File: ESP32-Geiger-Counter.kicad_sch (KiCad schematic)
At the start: 55 parts, among them J1 USB_C_Receptacle_USB2.0_16P, Q1 Q_NPN_BCE, Q2 Q_NPN_BCE, SW1 SW_Push, SW2 SW_Push, U1 TP4056-42-ESOP8, U2 USBLC6-2SC6, U3 ESP32-WROOM-32, U4 TPS63031DSK, U5 Geiger Mueller Tube, U6 CP2102N-Axx-xQFN24, U7 MC34063AD

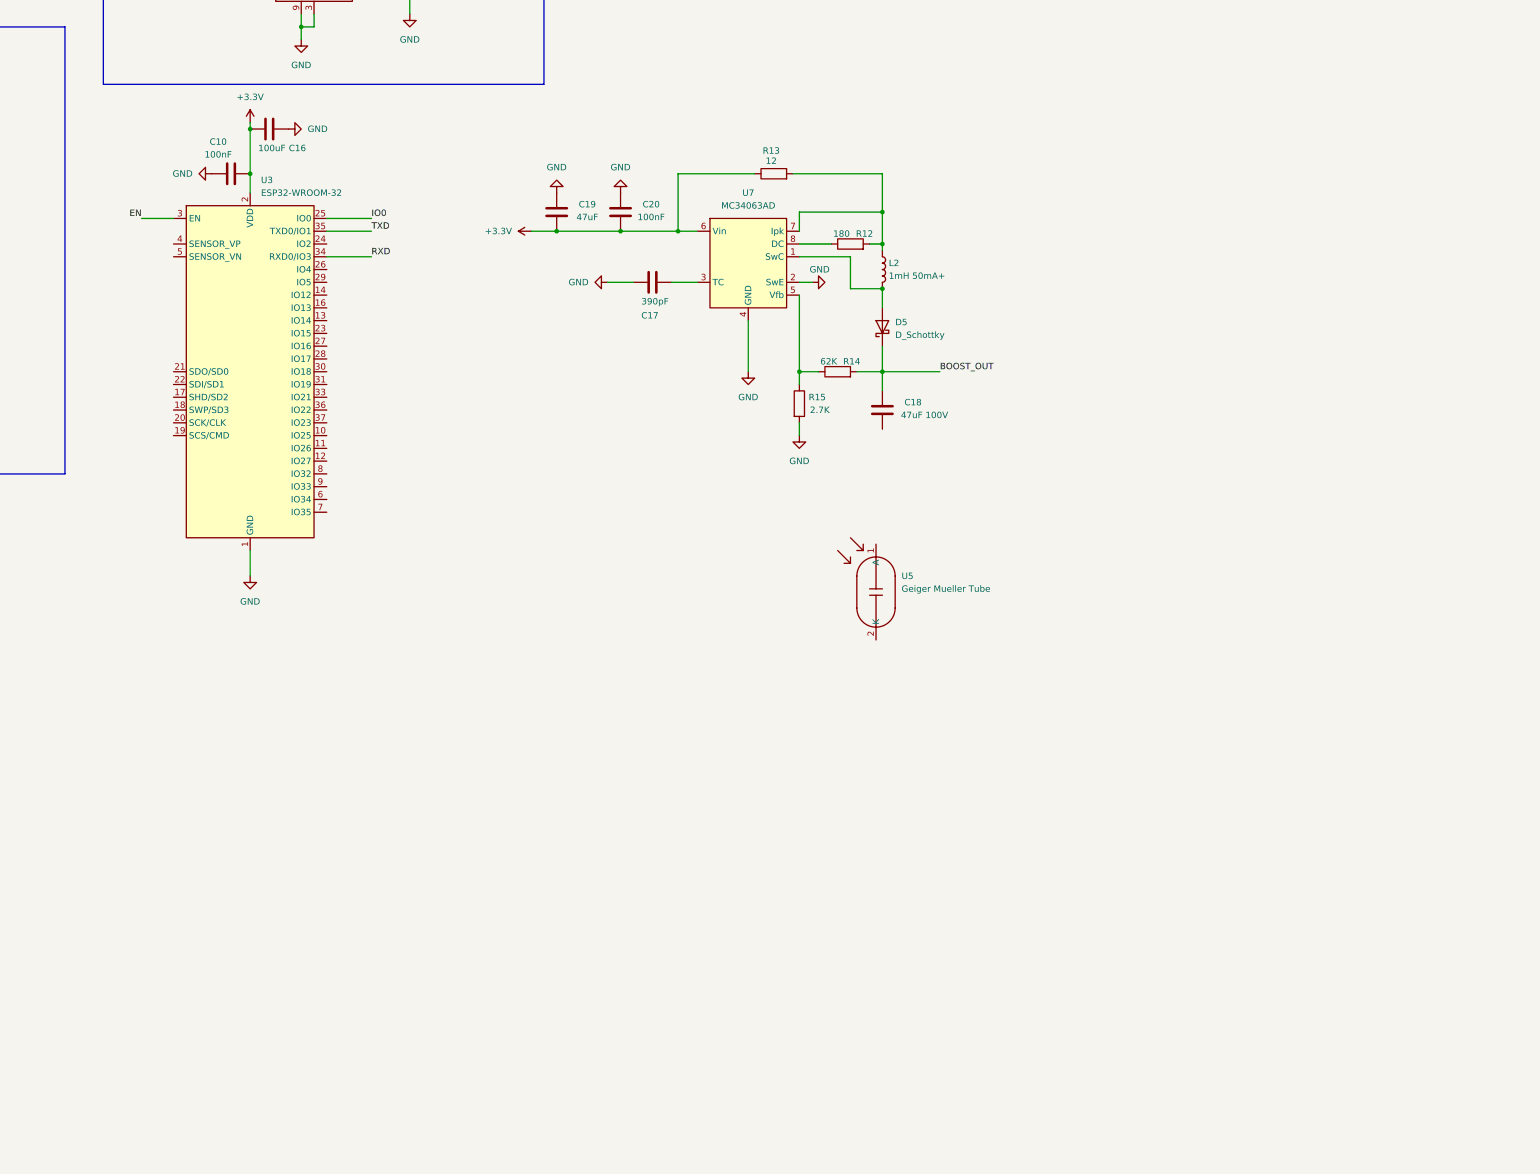
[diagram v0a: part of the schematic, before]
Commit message: idk if I will use this mega boost method
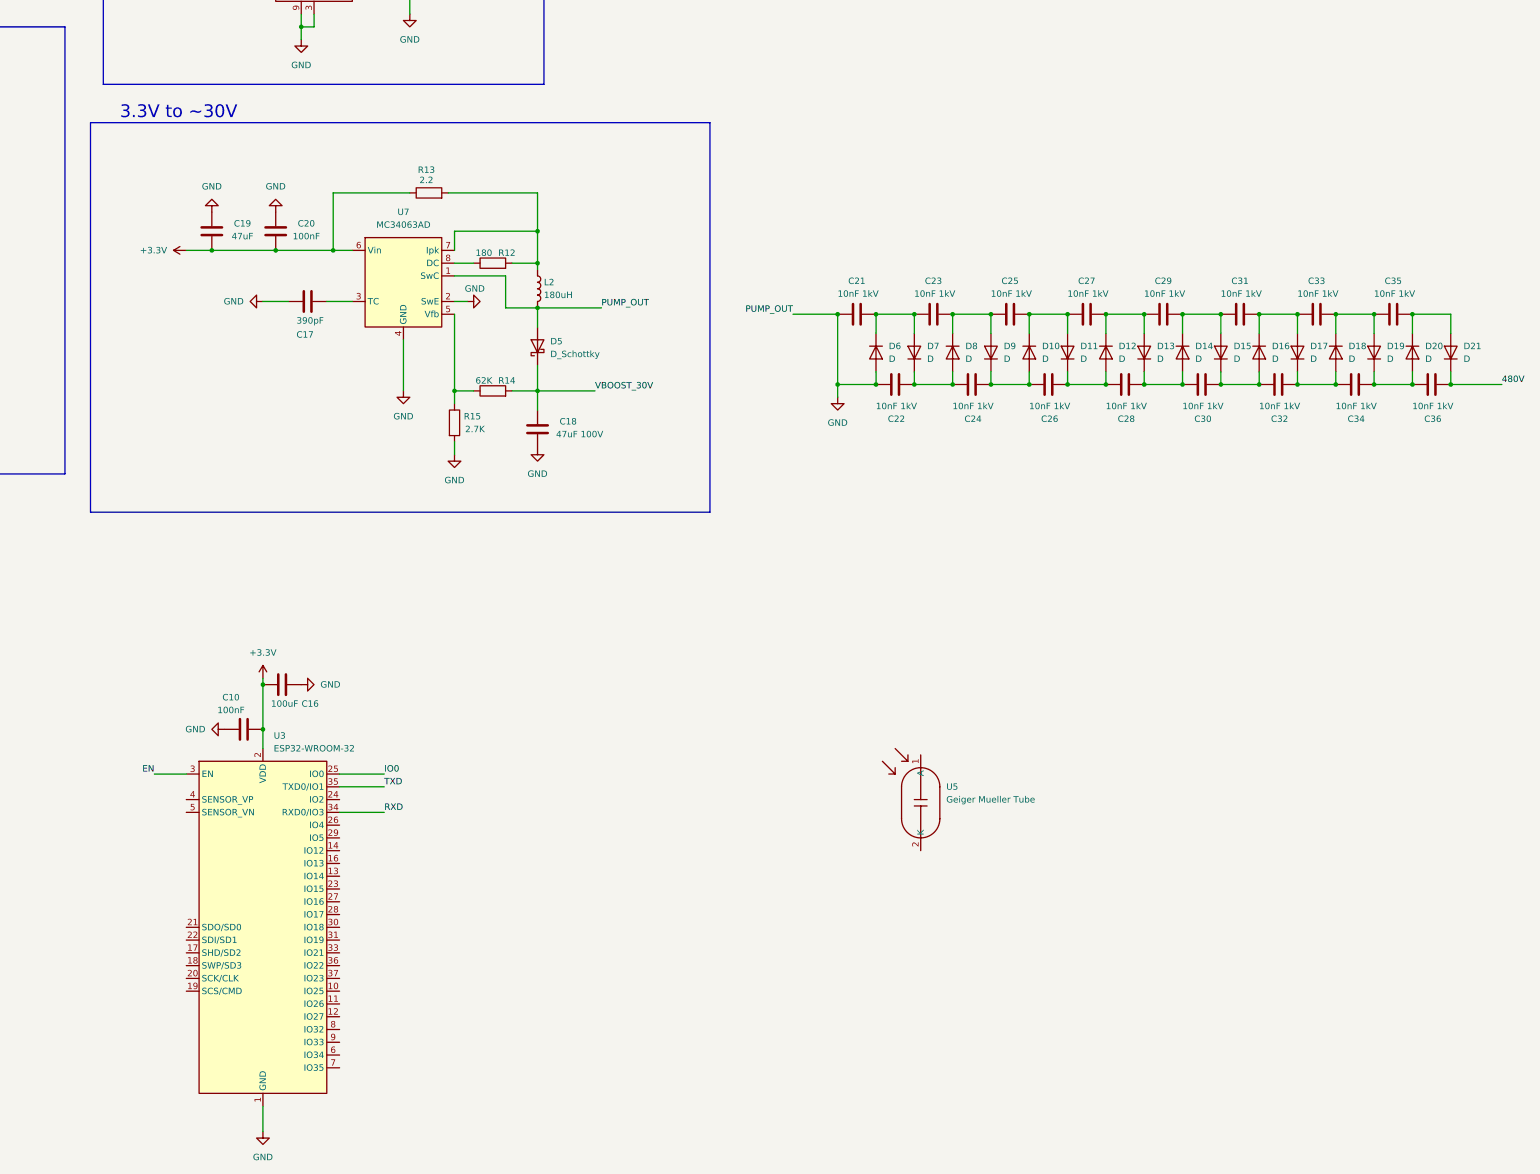
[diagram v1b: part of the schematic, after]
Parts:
- added C21, C22, C23, C24, C25, C26, C27, C28, C29, C30, C31, C32, C33, C34, C35, C36: 10nF 1kV, symbol Device:C
- added D10, D11, D12, D13, D14, D15, D16, D17, D18, D19, D20, D21, D6, D7, D8, D9: D, symbol Device:D
- L2: value 1mH 50mA+ -> 180uH
- R13: value 12 -> 2.2
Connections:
- net GND: now also C18.2, D5.2 (A), L2.2, U7.1 (SwC), C21.1, C22.1, D6.2 (A)
- net BOOST_OUT renamed VBOOST_30V
- new net: C21.2, C23.1, D6.1 (K), D7.2 (A)
- new net: C26.2, C28.1, D11.1 (K), D12.2 (A)
- new net: C25.2, C27.1, D10.1 (K), D11.2 (A)
- new net: C33.2, C35.1, D18.1 (K), D19.2 (A)
- new net: C32.2, C34.1, D17.1 (K), D18.2 (A)
- new net: C29.2, C31.1, D14.1 (K), D15.2 (A)
- new net: C28.2, C30.1, D13.1 (K), D14.2 (A)
- new net: C30.2, C32.1, D15.1 (K), D16.2 (A)
- new net: C35.2, D20.1 (K), D21.2 (A)
- new net: C34.2, C36.1, D19.1 (K), D20.2 (A)
- new net: C31.2, C33.1, D16.1 (K), D17.2 (A)
- new net: C22.2, C24.1, D7.1 (K), D8.2 (A)
- new net: C24.2, C26.1, D10.2 (A), D9.1 (K)
- new net: C23.2, C25.1, D8.1 (K), D9.2 (A)
- new net: C27.2, C29.1, D12.1 (K), D13.2 (A)
- new net 480V: C36.2, D21.1 (K)
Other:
- note added: "3.3V to ~30V"
- moved on the sheet: C10, C16, C17, C18, C19, C20, D5, L2, R12, R13, R14, R15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
